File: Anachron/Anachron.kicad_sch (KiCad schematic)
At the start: 0 parts

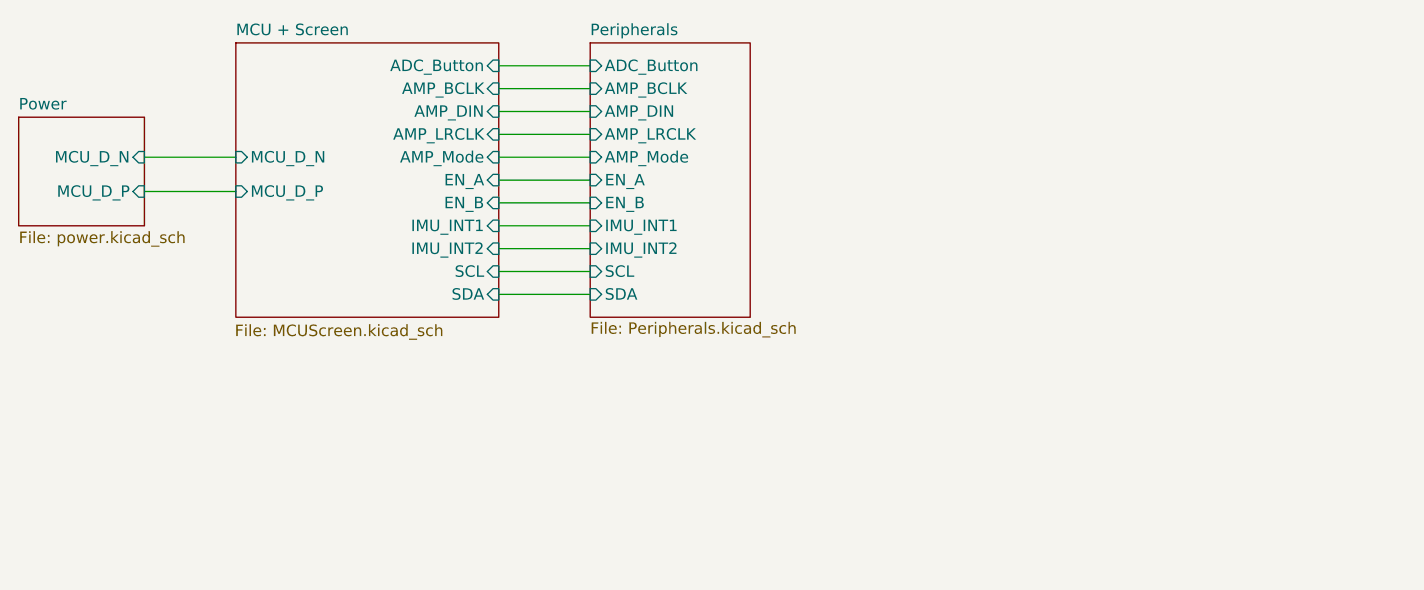
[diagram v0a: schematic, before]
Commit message: more changes!
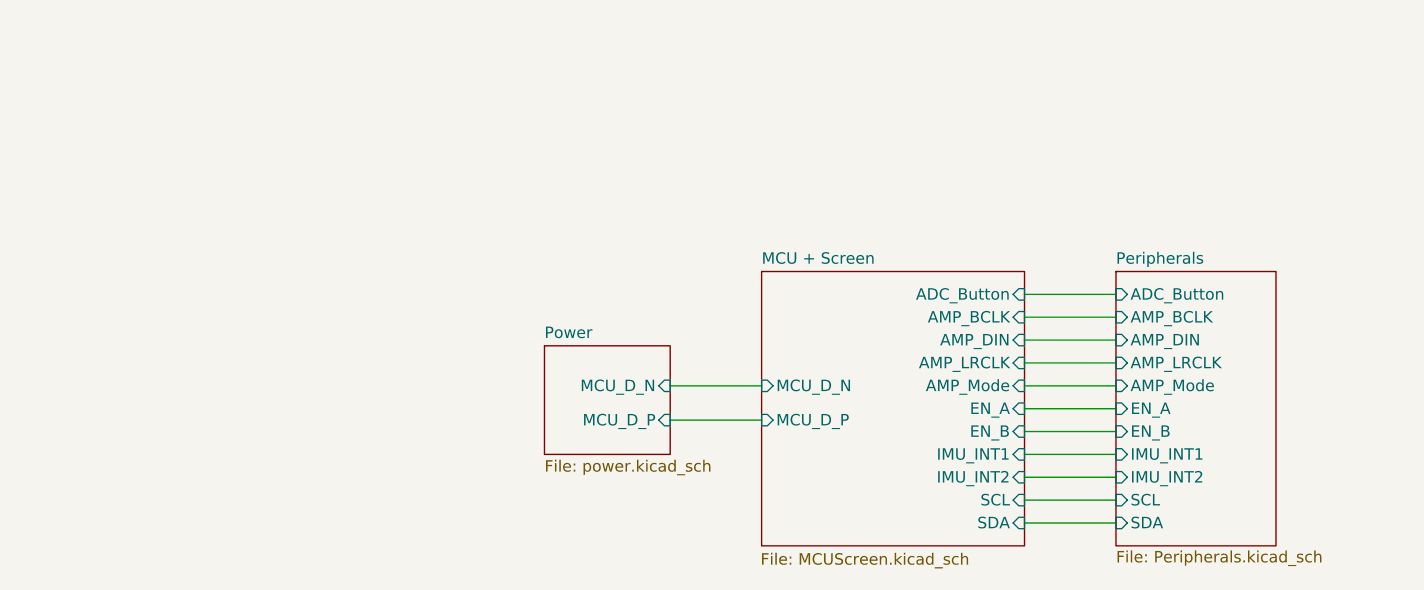
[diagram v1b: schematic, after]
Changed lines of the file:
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@@
 	(wire
 		(pts
-			(xy 63.5 63.5) (xy 73.66 63.5)
-		)
-		(stroke
-			(width 0)
-			(type default)
-		)
-	)
-	(wire
-		(pts
-			(xy 102.87 59.69) (xy 113.03 59.69)
-		)
-		(stroke
-			(width 0)
-			(type default)
-		)
-	)
-	(wire
-		(pts
-			(xy 63.5 59.69) (xy 73.66 59.69)
-		)
-		(stroke
-			(width 0)
-			(type default)
-		)
-	)
-	(wire
-		(pts
-			(xy 102.87 67.31) (xy 113.03 67.31)
-		)
-		(stroke
-			(width 0)
-			(type default)
-		)
-	)
-	(wire
-		(pts
-			(xy 102.87 69.85) (xy 113.03 69.85)
-		)
-		(stroke
-			(width 0)
-			(type default)
-		)
-	)
-	(wire
-		(pts
-			(xy 102.87 49.53) (xy 113.03 49.53)
-		)
-		(stroke
-			(width 0)
-			(type default)
-		)
-	)
-	(wire
-		(pts
-			(xy 102.87 72.39) (xy 113.03 72.39)
-		)
-		(stroke
-			(width 0)
-			(type default)
-		)
-	)
-	(wire
-		(pts
-			(xy 102.87 64.77) (xy 113.03 64.77)
-		)
-		(stroke
-			(width 0)
-			(type default)
-		)
-	)
-	(wire
-		(pts
-			(xy 102.87 57.15) (xy 113.03 57.15)
-		)
-		(stroke
-			(width 0)
-			(type default)
-		)
-	)
-	(wire
-		(pts
-			(xy 102.87 54.61) (xy 113.03 54.61)
-		)
-		(stroke
-			(width 0)
-			(type default)
-		)
-	)
-	(wire
-		(pts
-			(xy 102.87 52.07) (xy 113.03 52.07)
-		)
-		(stroke
-			(width 0)
-			(type default)
-		)
-	)
-	(wire
-		(pts
-			(xy 102.87 74.93) (xy 113.03 74.93)
-		)
-		(stroke
-			(width 0)
-			(type default)
-		)
-	)
-	(wire
-		(pts
-			(xy 102.87 62.23) (xy 113.03 62.23)
+			(xy 121.92 88.9) (xy 132.08 88.9)
+		)
+		(stroke
+			(width 0)
+			(type default)
+		)
+	)
+	(wire
+		(pts
+			(xy 161.29 85.09) (xy 171.45 85.09)
+		)
+		(stroke
+			(width 0)
+			(type default)
+		)
+	)
+	(wire
+		(pts
+			(xy 121.92 85.09) (xy 132.08 85.09)
+		)
+		(stroke
+			(width 0)
+			(type default)
+		)
+	)
+	(wire
+		(pts
+			(xy 161.29 92.71) (xy 171.45 92.71)
+		)
+		(stroke
+			(width 0)
+			(type default)
+		)
+	)
+	(wire
+		(pts
+			(xy 161.29 95.25) (xy 171.45 95.25)
+		)
+		(stroke
+			(width 0)
+			(type default)
+		)
+	)
+	(wire
+		(pts
+			(xy 161.29 74.93) (xy 171.45 74.93)
+		)
+		(stroke
+			(width 0)
+			(type default)
+		)
+	)
+	(wire
+		(pts
+			(xy 161.29 97.79) (xy 171.45 97.79)
+		)
+		(stroke
+			(width 0)
+			(type default)
+		)
+	)
+	(wire
+		(pts
+			(xy 161.29 90.17) (xy 171.45 90.17)
+		)
+		(stroke
+			(width 0)
+			(type default)
+		)
+	)
+	(wire
+		(pts
+			(xy 161.29 82.55) (xy 171.45 82.55)
+		)
+		(stroke
+			(width 0)
+			(type default)
+		)
+	)
+	(wire
+		(pts
+			(xy 161.29 80.01) (xy 171.45 80.01)
+		)
+		(stroke
+			(width 0)
+			(type default)
+		)
+	)
+	(wire
+		(pts
+			(xy 161.29 77.47) (xy 171.45 77.47)
+		)
+		(stroke
+			(width 0)
+			(type default)
+		)
+	)
+	(wire
+		(pts
+			(xy 161.29 100.33) (xy 171.45 100.33)
+		)
+		(stroke
+			(width 0)
+			(type default)
+		)
+	)
+	(wire
+		(pts
+			(xy 161.29 87.63) (xy 171.45 87.63)
 		)
 		(stroke
@@
 	)
 	(sheet
-		(at 73.66 46.99)
+		(at 132.08 72.39)
 		(size 29.21 30.48)
 		(exclude_from_sim no)
@@
 		)
 		(property "Sheetname" "MCU + Screen"
-			(at 73.66 46.2784 0)
+			(at 132.08 71.6784 0)
 			(show_name no)
 			(do_not_autoplace no)
@@
 		)
 		(property "Sheetfile" "MCUScreen.kicad_sch"
-			(at 73.533 78.232 0)
+			(at 131.953 103.632 0)
 			(show_name no)
 			(do_not_autoplace no)
@@
 		)
 		(pin "MCU_D_N" input
-			(at 73.66 59.69 180)
+			(at 132.08 85.09 180)
 			(effects
 				(font
@@
 		)
 		(pin "MCU_D_P" input
-			(at 73.66 63.5 180)
+			(at 132.08 88.9 180)
 			(effects
 				(font
@@
 		)
 		(pin "ADC_Button" input
-			(at 102.87 49.53 0)
+			(at 161.29 74.93 0)
 			(effects
 				(font
@@
 		)
 		(pin "AMP_BCLK" input
-			(at 102.87 52.07 0)
+			(at 161.29 77.47 0)
 			(effects
 				(font
@@
 		)
 		(pin "AMP_DIN" input
-			(at 102.87 54.61 0)
+			(at 161.29 80.01 0)
 			(effects
 				(font
@@
 		)
 		(pin "AMP_LRCLK" input
-			(at 102.87 57.15 0)
+			(at 161.29 82.55 0)
 			(effects
 				(font
@@
 		)
 		(pin "AMP_Mode" input
-			(at 102.87 59.69 0)
+			(at 161.29 85.09 0)
 			(effects
 				(font
@@
 		)
 		(pin "EN_A" input
-			(at 102.87 62.23 0)
+			(at 161.29 87.63 0)
 			(effects
 				(font
@@
 		)
 		(pin "EN_B" input
-			(at 102.87 64.77 0)
+			(at 161.29 90.17 0)
 			(effects
 				(font
@@
 		)
 		(pin "IMU_INT1" input
-			(at 102.87 67.31 0)
+			(at 161.29 92.71 0)
 			(effects
 				(font
@@
 		)
 		(pin "IMU_INT2" input
-			(at 102.87 69.85 0)
+			(at 161.29 95.25 0)
 			(effects
 				(font
@@
 		)
 		(pin "SCL" input
-			(at 102.87 72.39 0)
+			(at 161.29 97.79 0)
 			(effects
 				(font
@@
 		)
 		(pin "SDA" input
-			(at 102.87 74.93 0)
+			(at 161.29 100.33 0)
 			(effects
 				(font
@@
 	)
 	(sheet
-		(at 113.03 46.99)
+		(at 171.45 72.39)
 		(size 17.78 30.48)
 		(exclude_from_sim no)
@@
 		)
 		(property "Sheetname" "Peripherals"
-			(at 113.03 46.2784 0)
+			(at 171.45 71.6784 0)
 			(show_name no)
 			(do_not_autoplace no)
@@
 		)
 		(property "Sheetfile" "Peripherals.kicad_sch"
-			(at 113.03 77.978 0)
+			(at 171.45 103.378 0)
 			(show_name no)
 			(do_not_autoplace no)
@@
 		)
 		(pin "ADC_Button" input
-			(at 113.03 49.53 180)
+			(at 171.45 74.93 180)
 			(effects
 				(font
@@
 		)
 		(pin "AMP_BCLK" input
-			(at 113.03 52.07 180)
+			(at 171.45 77.47 180)
 			(effects
 				(font
@@
 		)
 		(pin "AMP_DIN" input
-			(at 113.03 54.61 180)
+			(at 171.45 80.01 180)
 			(effects
 				(font
@@
 		)
 		(pin "AMP_LRCLK" input
-			(at 113.03 57.15 180)
+			(at 171.45 82.55 180)
 			(effects
 				(font
@@
 		)
 		(pin "AMP_Mode" input
-			(at 113.03 59.69 180)
+			(at 171.45 85.09 180)
 			(effects
 				(font
@@
 		)
 		(pin "EN_A" input
-			(at 113.03 62.23 180)
+			(at 171.45 87.63 180)
 			(effects
 				(font
@@
 		)
 		(pin "EN_B" input
-			(at 113.03 64.77 180)
+			(at 171.45 90.17 180)
 			(effects
 				(font
@@
 		)
 		(pin "IMU_INT1" input
-			(at 113.03 67.31 180)
+			(at 171.45 92.71 180)
 			(effects
 				(font
@@
 		)
 		(pin "IMU_INT2" input
-			(at 113.03 69.85 180)
+			(at 171.45 95.25 180)
 			(effects
 				(font
@@
 		)
 		(pin "SCL" input
-			(at 113.03 72.39 180)
+			(at 171.45 97.79 180)
 			(effects
 				(font
@@
 		)
 		(pin "SDA" input
-			(at 113.03 74.93 180)
+			(at 171.45 100.33 180)
 			(effects
 				(font
@@
 	)
 	(sheet
-		(at 49.53 55.245)
+		(at 107.95 80.645)
 		(size 13.97 12.065)
 		(exclude_from_sim no)
@@
 		)
 		(property "Sheetname" "Power"
-			(at 49.53 54.5334 0)
+			(at 107.95 79.9334 0)
 			(show_name no)
 			(do_not_autoplace no)
@@
 		)
 		(property "Sheetfile" "power.kicad_sch"
-			(at 49.53 67.8946 0)
+			(at 107.95 93.2946 0)
 			(show_name no)
 			(do_not_autoplace no)
@@
 		)
 		(pin "MCU_D_N" input
-			(at 63.5 59.69 0)
+			(at 121.92 85.09 0)
 			(effects
 				(font
@@
 		)
 		(pin "MCU_D_P" input
-			(at 63.5 63.5 0)
-			(effects
-				(font
+			(at 121.92 88.9 0)
+			(effects
+				(font
